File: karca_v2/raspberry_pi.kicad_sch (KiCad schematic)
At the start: 9 parts, among them J7 Raspberry_pi, Q2 PN2222A, U11 M41T93

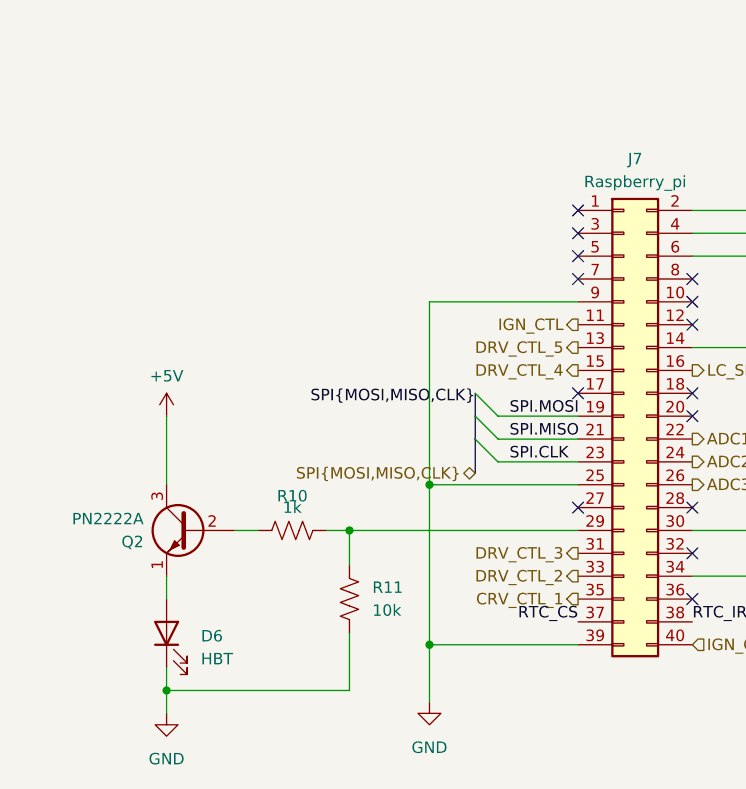
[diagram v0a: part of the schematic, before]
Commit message: fkkkkkkkkkk
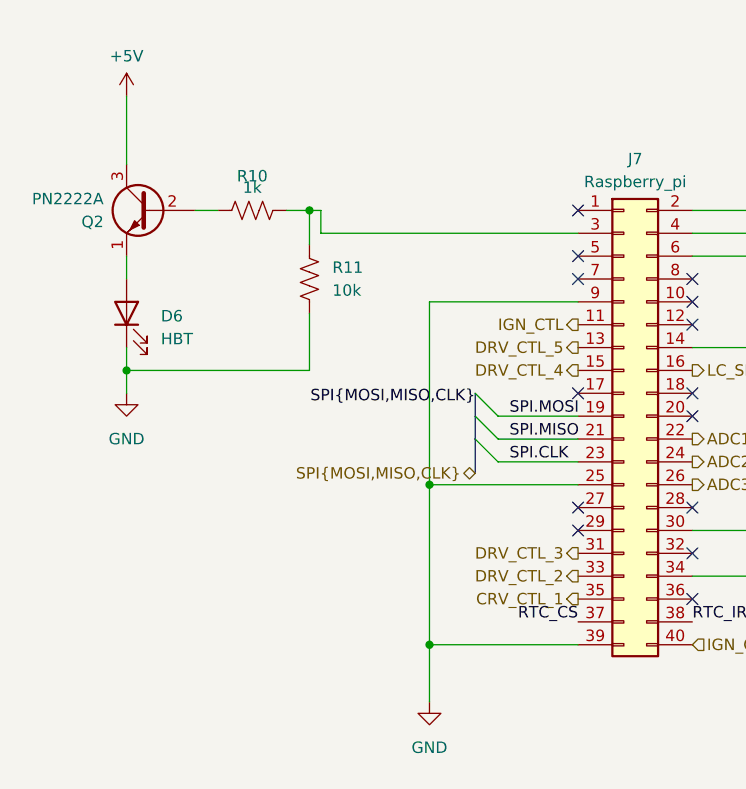
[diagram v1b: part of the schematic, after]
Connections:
- net at R10.2, R11.2: now also J7.3 (Pin_3); no longer J7.29 (Pin_29)
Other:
- moved on the sheet: D6, Q2, R10, R11
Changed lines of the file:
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@@
   (junction (at 160.02 60.96) (diameter 0) (color 0 0 0 0)
   )
+  (junction (at 108.585 60.96) (diameter 0) (color 0 0 0 0)
+  )
   (junction (at 121.92 91.44) (diameter 0) (color 0 0 0 0)
   )
@@
   (junction (at 121.92 109.22) (diameter 0) (color 0 0 0 0)
   )
-  (junction (at 113.03 96.52) (diameter 0) (color 0 0 0 0)
-  )
   (junction (at 215.9 60.96) (diameter 0) (color 0 0 0 0)
   )
@@
   (junction (at 195.58 60.96) (diameter 0) (color 0 0 0 0)
   )
-  (junction (at 92.71 114.3) (diameter 0) (color 0 0 0 0)
+  (junction (at 88.265 78.74) (diameter 0) (color 0 0 0 0)
   )
   (no_connect (at 151.13 73.66))
+  (no_connect (at 138.43 96.52))
   (no_connect (at 198.12 71.12))
   (no_connect (at 151.13 104.14))
-  (no_connect (at 138.43 63.5))
   (no_connect (at 138.43 68.58))
   (no_connect (at 151.13 83.82))
@@
     (stroke (width 0) (type default))
   )
+  (wire (pts (xy 109.855 63.5) (xy 109.855 60.96))
+    (stroke (width 0) (type default))
+  )
   (wire (pts (xy 160.02 63.5) (xy 160.02 60.96))
     (stroke (width 0) (type default))
   )
-  (wire (pts (xy 113.03 96.52) (xy 113.03 100.33))
+  (wire (pts (xy 108.585 60.96) (xy 108.585 64.77))
     (stroke (width 0) (type default))
   )
@@
     (stroke (width 0) (type default))
   )
-  (wire (pts (xy 100.33 96.52) (xy 102.87 96.52))
+  (wire (pts (xy 95.885 60.96) (xy 98.425 60.96))
     (stroke (width 0) (type default))
   )
@@
     (stroke (width 0) (type default))
   )
-  (wire (pts (xy 92.71 111.76) (xy 92.71 114.3))
-    (stroke (width 0) (type default))
-  )
-  (wire (pts (xy 92.71 114.3) (xy 92.71 116.84))
+  (wire (pts (xy 88.265 76.2) (xy 88.265 78.74))
+    (stroke (width 0) (type default))
+  )
+  (wire (pts (xy 88.265 78.74) (xy 88.265 81.28))
     (stroke (width 0) (type default))
   )
@@
     (stroke (width 0) (type default))
   )
-  (wire (pts (xy 113.03 114.3) (xy 92.71 114.3))
-    (stroke (width 0) (type default))
-  )
-  (wire (pts (xy 113.03 107.95) (xy 113.03 114.3))
+  (wire (pts (xy 108.585 78.74) (xy 88.265 78.74))
+    (stroke (width 0) (type default))
+  )
+  (wire (pts (xy 108.585 72.39) (xy 108.585 78.74))
     (stroke (width 0) (type default))
   )
@@
     (stroke (width 0) (type default))
   )
+  (wire (pts (xy 109.855 60.96) (xy 108.585 60.96))
+    (stroke (width 0) (type default))
+  )
   (wire (pts (xy 121.92 91.44) (xy 138.43 91.44))
     (stroke (width 0) (type default))
@@
     (stroke (width 0) (type default))
   )
-  (wire (pts (xy 113.03 96.52) (xy 110.49 96.52))
+  (wire (pts (xy 108.585 60.96) (xy 106.045 60.96))
     (stroke (width 0) (type default))
   )
@@
     (stroke (width 0) (type default))
   )
-  (wire (pts (xy 92.71 101.6) (xy 92.71 104.14))
+  (wire (pts (xy 88.265 66.04) (xy 88.265 68.58))
     (stroke (width 0) (type default))
   )
@@
     (stroke (width 0) (type default))
   )
-  (wire (pts (xy 92.71 83.82) (xy 92.71 91.44))
+  (wire (pts (xy 88.265 48.26) (xy 88.265 55.88))
     (stroke (width 0) (type default))
   )
@@
     (stroke (width 0) (type default))
   )
-  (wire (pts (xy 113.03 96.52) (xy 138.43 96.52))
-    (stroke (width 0) (type default))
-  )
   (wire (pts (xy 198.12 76.2) (xy 195.58 76.2))
     (stroke (width 0) (type default))
@@
   )
   (wire (pts (xy 121.92 109.22) (xy 121.92 115.57))
+    (stroke (width 0) (type default))
+  )
+  (wire (pts (xy 138.43 63.5) (xy 109.855 63.5))
     (stroke (width 0) (type default))
   )
@@
     )
   )
-  (symbol (lib_id "Device:R_US") (at 113.03 104.14 180) (unit 1)
-    (in_bom yes) (on_board yes) (dnp no) (fields_autoplaced)
-    (property "Reference" "R11" (at 115.57 102.87 0)
+  (symbol (lib_id "Device:R_US") (at 108.585 68.58 180) (unit 1)
+    (in_bom yes) (on_board yes) (dnp no) (fields_autoplaced)
+    (property "Reference" "R11" (at 111.125 67.31 0)
       (effects (font (size 1.27 1.27)) (justify right))
     )
-    (property "Value" "10k" (at 115.57 105.41 0)
+    (property "Value" "10k" (at 111.125 69.85 0)
       (effects (font (size 1.27 1.27)) (justify right))
     )
-    (property "Footprint" "Resistor_SMD:R_1206_3216Metric" (at 112.014 103.886 90)
-      (effects (font (size 1.27 1.27)) hide)
-    )
-    (property "Datasheet" "~" (at 113.03 104.14 0)
+    (property "Footprint" "Resistor_SMD:R_1206_3216Metric" (at 107.569 68.326 90)
+      (effects (font (size 1.27 1.27)) hide)
+    )
+    (property "Datasheet" "~" (at 108.585 68.58 0)
       (effects (font (size 1.27 1.27)) hide)
     )
@@
     )
   )
-  (symbol (lib_id "Device:R_US") (at 106.68 96.52 90) (unit 1)
+  (symbol (lib_id "Device:R_US") (at 102.235 60.96 90) (unit 1)
     (in_bom yes) (on_board yes) (dnp no)
-    (property "Reference" "R10" (at 106.68 92.71 90)
-      (effects (font (size 1.27 1.27)))
-    )
-    (property "Value" "1k" (at 106.68 93.98 90)
-      (effects (font (size 1.27 1.27)))
-    )
-    (property "Footprint" "Resistor_SMD:R_1206_3216Metric" (at 106.934 95.504 90)
-      (effects (font (size 1.27 1.27)) hide)
-    )
-    (property "Datasheet" "~" (at 106.68 96.52 0)
+    (property "Reference" "R10" (at 102.235 57.15 90)
+      (effects (font (size 1.27 1.27)))
+    )
+    (property "Value" "1k" (at 102.235 58.42 90)
+      (effects (font (size 1.27 1.27)))
+    )
+    (property "Footprint" "Resistor_SMD:R_1206_3216Metric" (at 102.489 59.944 90)
+      (effects (font (size 1.27 1.27)) hide)
+    )
+    (property "Datasheet" "~" (at 102.235 60.96 0)
       (effects (font (size 1.27 1.27)) hide)
     )
@@
     )
   )
-  (symbol (lib_id "Device:LED") (at 92.71 107.95 90) (unit 1)
-    (in_bom yes) (on_board yes) (dnp no) (fields_autoplaced)
-    (property "Reference" "D6" (at 96.52 108.2675 90)
+  (symbol (lib_id "Device:LED") (at 88.265 72.39 90) (unit 1)
+    (in_bom yes) (on_board yes) (dnp no) (fields_autoplaced)
+    (property "Reference" "D6" (at 92.075 72.7075 90)
       (effects (font (size 1.27 1.27)) (justify right))
     )
-    (property "Value" "HBT" (at 96.52 110.8075 90)
+    (property "Value" "HBT" (at 92.075 75.2475 90)
       (effects (font (size 1.27 1.27)) (justify right))
     )
-    (property "Footprint" "LED_SMD:LED_1206_3216Metric" (at 92.71 107.95 0)
-      (effects (font (size 1.27 1.27)) hide)
-    )
-    (property "Datasheet" "~" (at 92.71 107.95 0)
+    (property "Footprint" "LED_SMD:LED_1206_3216Metric" (at 88.265 72.39 0)
+      (effects (font (size 1.27 1.27)) hide)
+    )
+    (property "Datasheet" "~" (at 88.265 72.39 0)
       (effects (font (size 1.27 1.27)) hide)
     )
@@
     )
   )
-  (symbol (lib_id "Transistor_BJT:PN2222A") (at 95.25 96.52 0) (mirror y) (unit 1)
+  (symbol (lib_id "Transistor_BJT:PN2222A") (at 90.805 60.96 0) (mirror y) (unit 1)
     (in_bom yes) (on_board yes) (dnp no)
-    (property "Reference" "Q2" (at 90.17 97.79 0)
+    (property "Reference" "Q2" (at 85.725 62.23 0)
       (effects (font (size 1.27 1.27)) (justify left))
     )
-    (property "Value" "PN2222A" (at 90.17 95.25 0)
+    (property "Value" "PN2222A" (at 85.725 59.69 0)
       (effects (font (size 1.27 1.27)) (justify left))
     )
-    (property "Footprint" "Package_TO_SOT_THT:TO-92_Inline" (at 90.17 98.425 0)
+    (property "Footprint" "Package_TO_SOT_THT:TO-92_Inline" (at 85.725 62.865 0)
       (effects (font (size 1.27 1.27) italic) (justify left) hide)
     )
-    (property "Datasheet" "https://www.onsemi.com/pub/Collateral/PN2222-D.PDF" (at 95.25 96.52 0)
+    (property "Datasheet" "https://www.onsemi.com/pub/Collateral/PN2222-D.PDF" (at 90.805 60.96 0)
       (effects (font (size 1.27 1.27)) (justify left) hide)
     )
@@
     )
   )
-  (symbol (lib_id "power:GND") (at 92.71 116.84 0) (unit 1)
-    (in_bom yes) (on_board yes) (dnp no) (fields_autoplaced)
-    (property "Reference" "#PWR046" (at 92.71 123.19 0)
-      (effects (font (size 1.27 1.27)) hide)
-    )
-    (property "Value" "GND" (at 92.71 121.92 0)
-      (effects (font (size 1.27 1.27)))
-    )
-    (property "Footprint" "" (at 92.71 116.84 0)
-      (effects (font (size 1.27 1.27)) hide)
-    )
-    (property "Datasheet" "" (at 92.71 116.84 0)
+  (symbol (lib_id "power:GND") (at 88.265 81.28 0) (unit 1)
+    (in_bom yes) (on_board yes) (dnp no) (fields_autoplaced)
+    (property "Reference" "#PWR046" (at 88.265 87.63 0)
+      (effects (font (size 1.27 1.27)) hide)
+    )
+    (property "Value" "GND" (at 88.265 86.36 0)
+      (effects (font (size 1.27 1.27)))
+    )
+    (property "Footprint" "" (at 88.265 81.28 0)
+      (effects (font (size 1.27 1.27)) hide)
+    )
+    (property "Datasheet" "" (at 88.265 81.28 0)
       (effects (font (size 1.27 1.27)) hide)
     )
@@
     )
   )
-  (symbol (lib_id "power:+5V") (at 92.71 83.82 0) (unit 1)
-    (in_bom yes) (on_board yes) (dnp no) (fields_autoplaced)
-    (property "Reference" "#PWR042" (at 92.71 87.63 0)
-      (effects (font (size 1.27 1.27)) hide)
-    )
-    (property "Value" "+5V" (at 92.71 79.375 0)
-      (effects (font (size 1.27 1.27)))
-    )
-    (property "Footprint" "" (at 92.71 83.82 0)
-      (effects (font (size 1.27 1.27)) hide)
-    )
-    (property "Datasheet" "" (at 92.71 83.82 0)
-      (effects (font (size 1.27 1.27)) hide)
-    )
+  (symbol (lib_id "power:+5V") (at 88.265 48.26 0) (unit 1)
+    (in_bom yes) (on_board yes) (dnp no) (fields_autoplaced)
+    (property "Reference" "#PWR042" (at 88.265 52.07 0)
+      (effects (font (size 1.27 1.27)) hide)
+    )
+    (property "Value" "+5V" (at 88.265 43.815 0)
+      (effects (font (size 1.27 1.27)))
+    )
+    (property "Footprint" "" (at 88.265 48.26 0)
+      (effects (font (size 1.27 1.27)) hide)
+    )
+    (property "Datasheet" "" (at 88.265 48.26 0)
+      (effects (font (size 1.27 1.27)) hide)
+    )
